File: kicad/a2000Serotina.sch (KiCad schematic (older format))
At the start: 23 parts

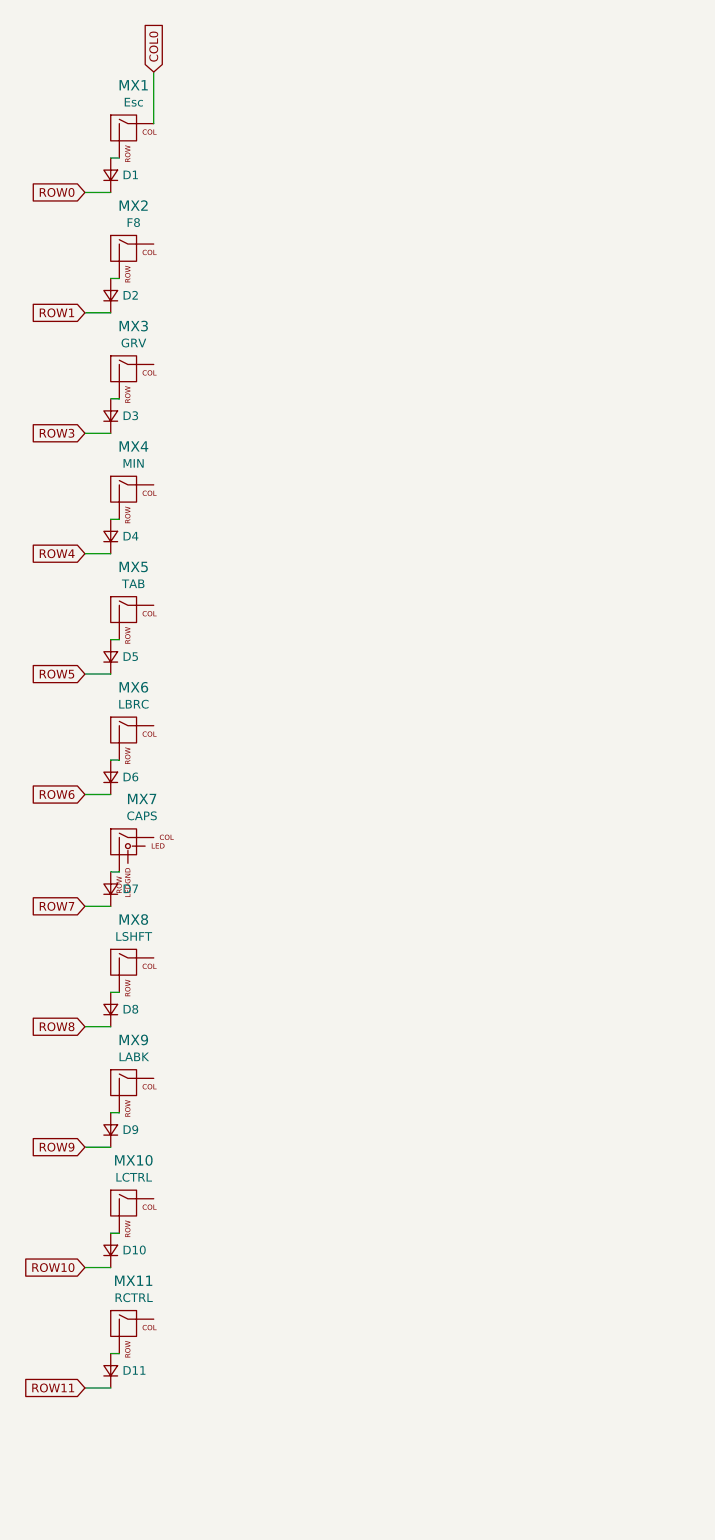
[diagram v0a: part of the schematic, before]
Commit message: Further work on Keyboard Matrix
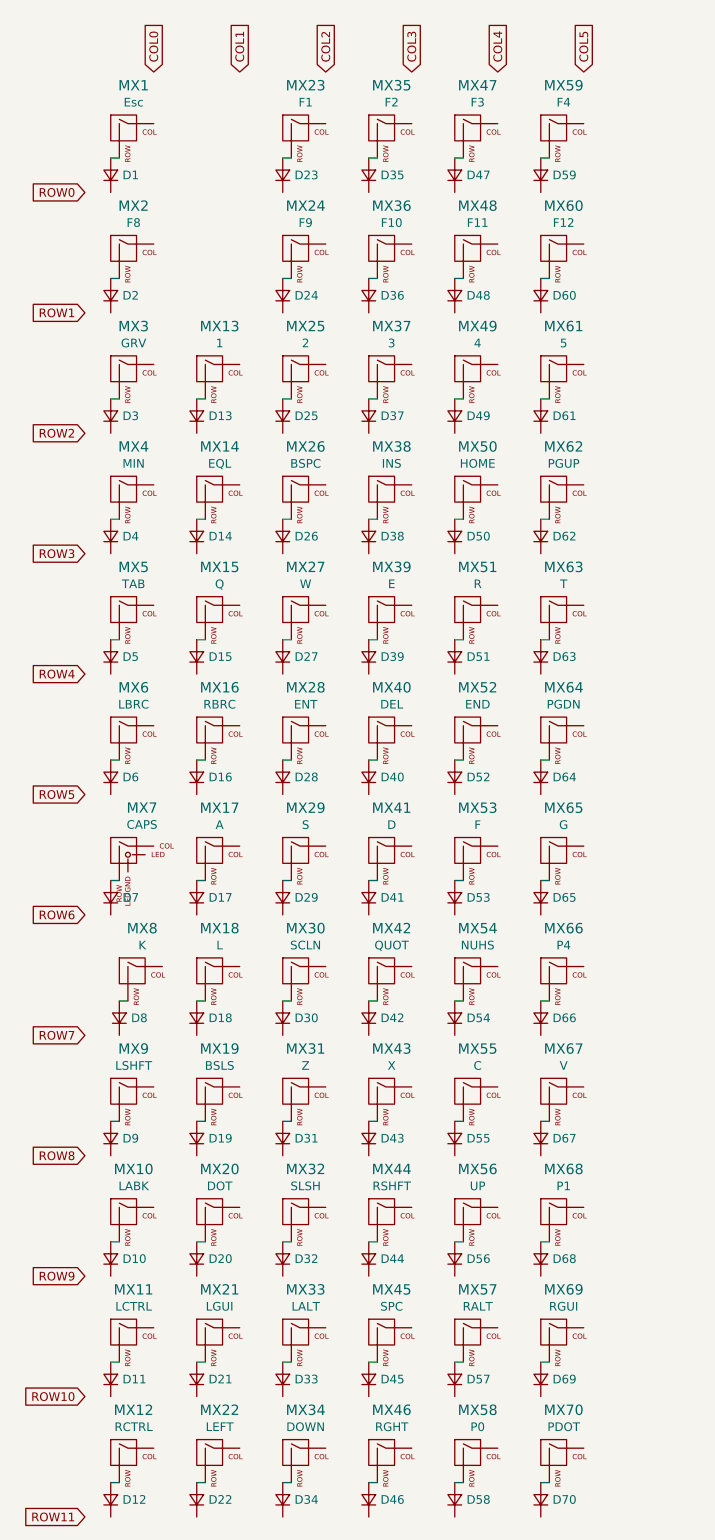
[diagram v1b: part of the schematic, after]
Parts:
- added D13, D14, D15, D16, D17, D18, D19, D20, D21, D22, D23, D24, D25, D26, D27, D28, D29, D30, D31, D32, D33, D34, D35, D36, D37, D38, D39, D40, D41, D42, D43, D44, D45, D46, D47, D48, D49, D50, D51, D52, D53, D54, D55, D56, D57, D58, D59, D60, D61, D62, D63, D64, D65, D66, D67, D68, D69, D70, D8: D_Small, symbol Device:D_Small
- added MX13, MX14, MX15, MX16, MX17, MX18, MX19, MX20, MX21, MX22, MX23, MX24, MX25, MX26, MX27, MX28, MX29, MX30, MX31, MX32, MX33, MX34, MX35, MX36, MX37, MX38, MX39, MX40, MX41, MX42, MX43, MX44, MX45, MX46, MX47, MX48, MX49, MX50, MX51, MX52, MX53, MX54, MX55, MX56, MX57, MX58, MX59, MX60, MX61, MX62, MX63, MX64, MX65, MX66, MX67, MX68, MX69, MX70, MX8: MX-NoLED, symbol MX_Alps_Hybrid:MX-NoLED
- renumbered D9 to D10, D10 to D11, D11 to D12, D8 to D9, MX9 to MX10, MX10 to MX11, MX11 to MX12, MX8 to MX9
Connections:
- net COL0: no longer MX1.1 (COL)
- net ROW0: no longer D1.1 (K)
- net ROW1: no longer D2.1 (K)
- net ROW10: no longer D11.1 (K)
- net ROW11: no longer D12.1 (K)
- net ROW3: no longer D3.1 (K)
- net ROW4: no longer D4.1 (K)
- net ROW5: no longer D5.1 (K)
- net ROW6: no longer D6.1 (K)
- net ROW7: no longer D7.1 (K)
- net ROW8: no longer D9.1 (K)
- net ROW9: no longer D10.1 (K)
- new net: D13.2 (A), MX13.2 (ROW)
- new net: D14.2 (A), MX14.2 (ROW)
- new net: D15.2 (A), MX15.2 (ROW)
- new net: D16.2 (A), MX16.2 (ROW)
- new net: D17.2 (A), MX17.2 (ROW)
- new net: D19.2 (A), MX19.2 (ROW)
- new net: D20.2 (A), MX20.2 (ROW)
- new net: D21.2 (A), MX21.2 (ROW)
- new net: D22.2 (A), MX22.2 (ROW)
- new net: D25.2 (A), MX25.2 (ROW)
- new net: D24.2 (A), MX24.2 (ROW)
- new net: D23.2 (A), MX23.2 (ROW)
- new net: D26.2 (A), MX26.2 (ROW)
- new net: D27.2 (A), MX27.2 (ROW)
- new net: D28.2 (A), MX28.2 (ROW)
- new net: D29.2 (A), MX29.2 (ROW)
- new net: D30.2 (A), MX30.2 (ROW)
- new net: D31.2 (A), MX31.2 (ROW)
- new net: D18.2 (A), MX18.2 (ROW)
- new net: D8.2 (A), MX8.2 (ROW)
- new net: D32.2 (A), MX32.2 (ROW)
- new net: D33.2 (A), MX33.2 (ROW)
- new net: D34.2 (A), MX34.2 (ROW)
- new net: D35.2 (A), MX35.2 (ROW)
- new net: D36.2 (A), MX36.2 (ROW)
- new net: D37.2 (A), MX37.2 (ROW)
- new net: D38.2 (A), MX38.2 (ROW)
- new net: D39.2 (A), MX39.2 (ROW)
- new net: D40.2 (A), MX40.2 (ROW)
- new net: D41.2 (A), MX41.2 (ROW)
- new net: D42.2 (A), MX42.2 (ROW)
- new net: D43.2 (A), MX43.2 (ROW)
- new net: D44.2 (A), MX44.2 (ROW)
- new net: D45.2 (A), MX45.2 (ROW)
- new net: D46.2 (A), MX46.2 (ROW)
- new net: D47.2 (A), MX47.2 (ROW)
- new net: D48.2 (A), MX48.2 (ROW)
- new net: D49.2 (A), MX49.2 (ROW)
- new net: D50.2 (A), MX50.2 (ROW)
- new net: D51.2 (A), MX51.2 (ROW)
- new net: D52.2 (A), MX52.2 (ROW)
- new net: D53.2 (A), MX53.2 (ROW)
- new net: D54.2 (A), MX54.2 (ROW)
- new net: D55.2 (A), MX55.2 (ROW)
- new net: D56.2 (A), MX56.2 (ROW)
- new net: D57.2 (A), MX57.2 (ROW)
- new net: D58.2 (A), MX58.2 (ROW)
- new net: D59.2 (A), MX59.2 (ROW)
- new net: D60.2 (A), MX60.2 (ROW)
- new net: D61.2 (A), MX61.2 (ROW)
- new net: D62.2 (A), MX62.2 (ROW)
- new net: D63.2 (A), MX63.2 (ROW)
- new net: D64.2 (A), MX64.2 (ROW)
- new net: D65.2 (A), MX65.2 (ROW)
- new net: D66.2 (A), MX66.2 (ROW)
- new net: D67.2 (A), MX67.2 (ROW)
- new net: D68.2 (A), MX68.2 (ROW)
- new net: D69.2 (A), MX69.2 (ROW)
- new net: D70.2 (A), MX70.2 (ROW)
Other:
- moved on the sheet: D10, D11, D12, D7, D9, MX10, MX11, MX12, MX7, MX9

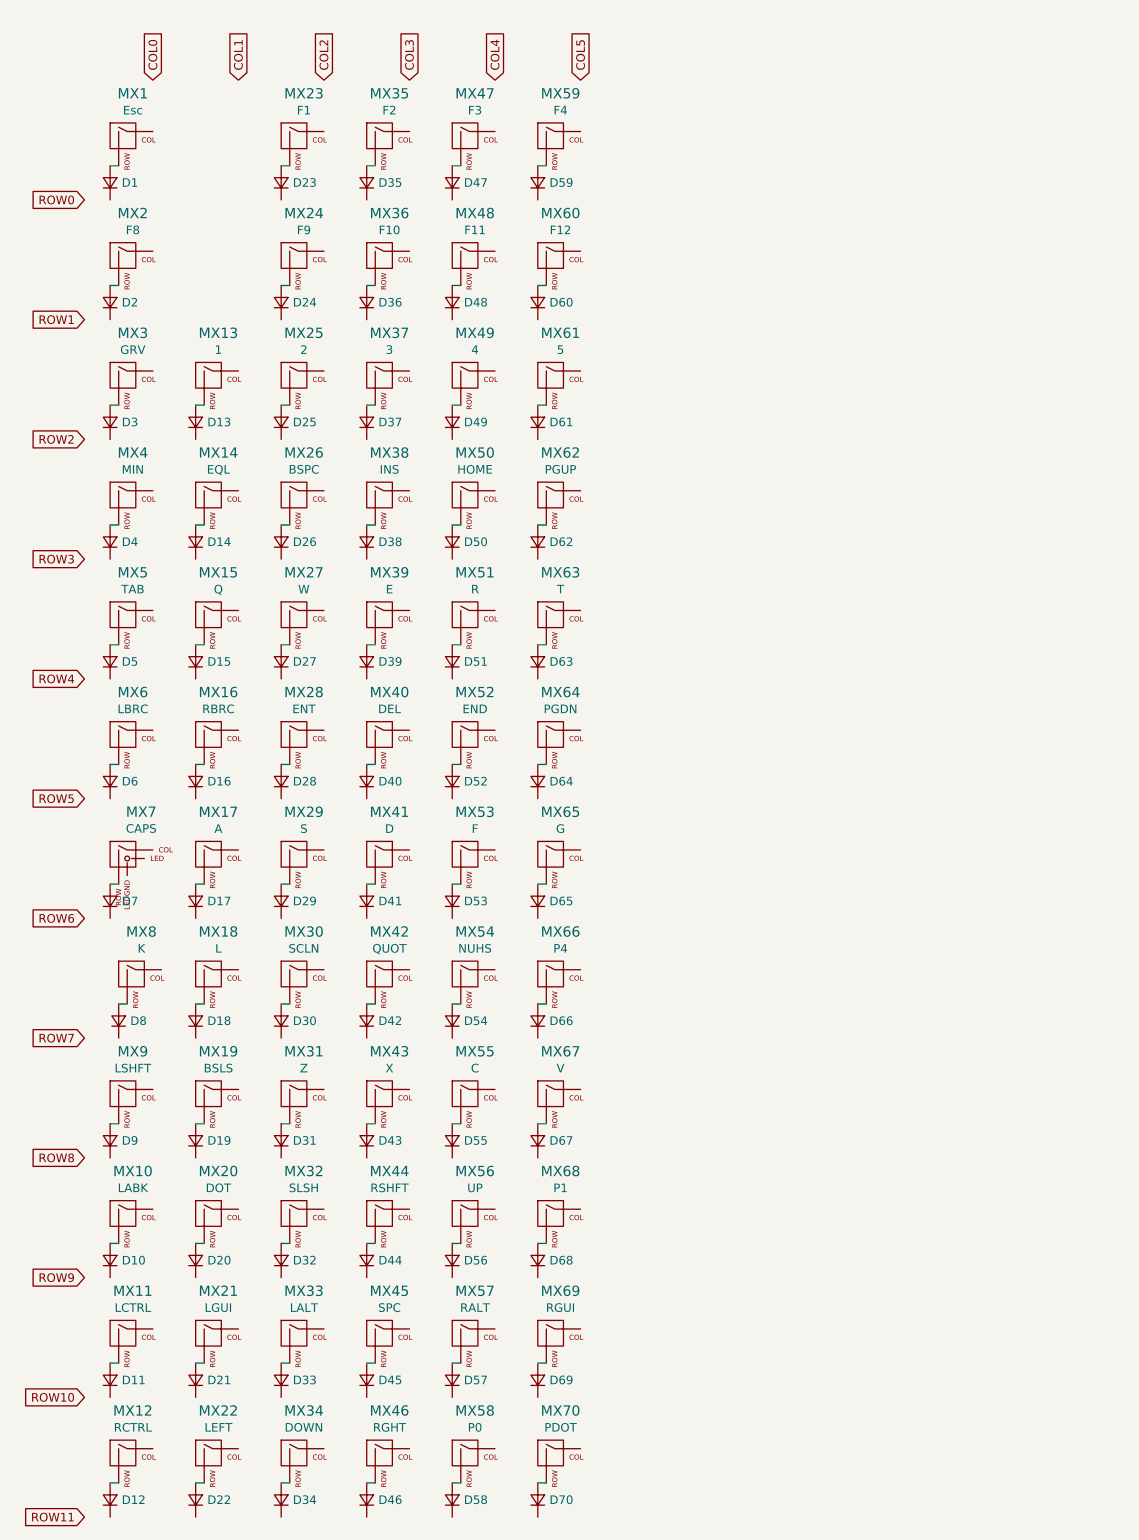
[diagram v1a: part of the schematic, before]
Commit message: Matrix now complete.
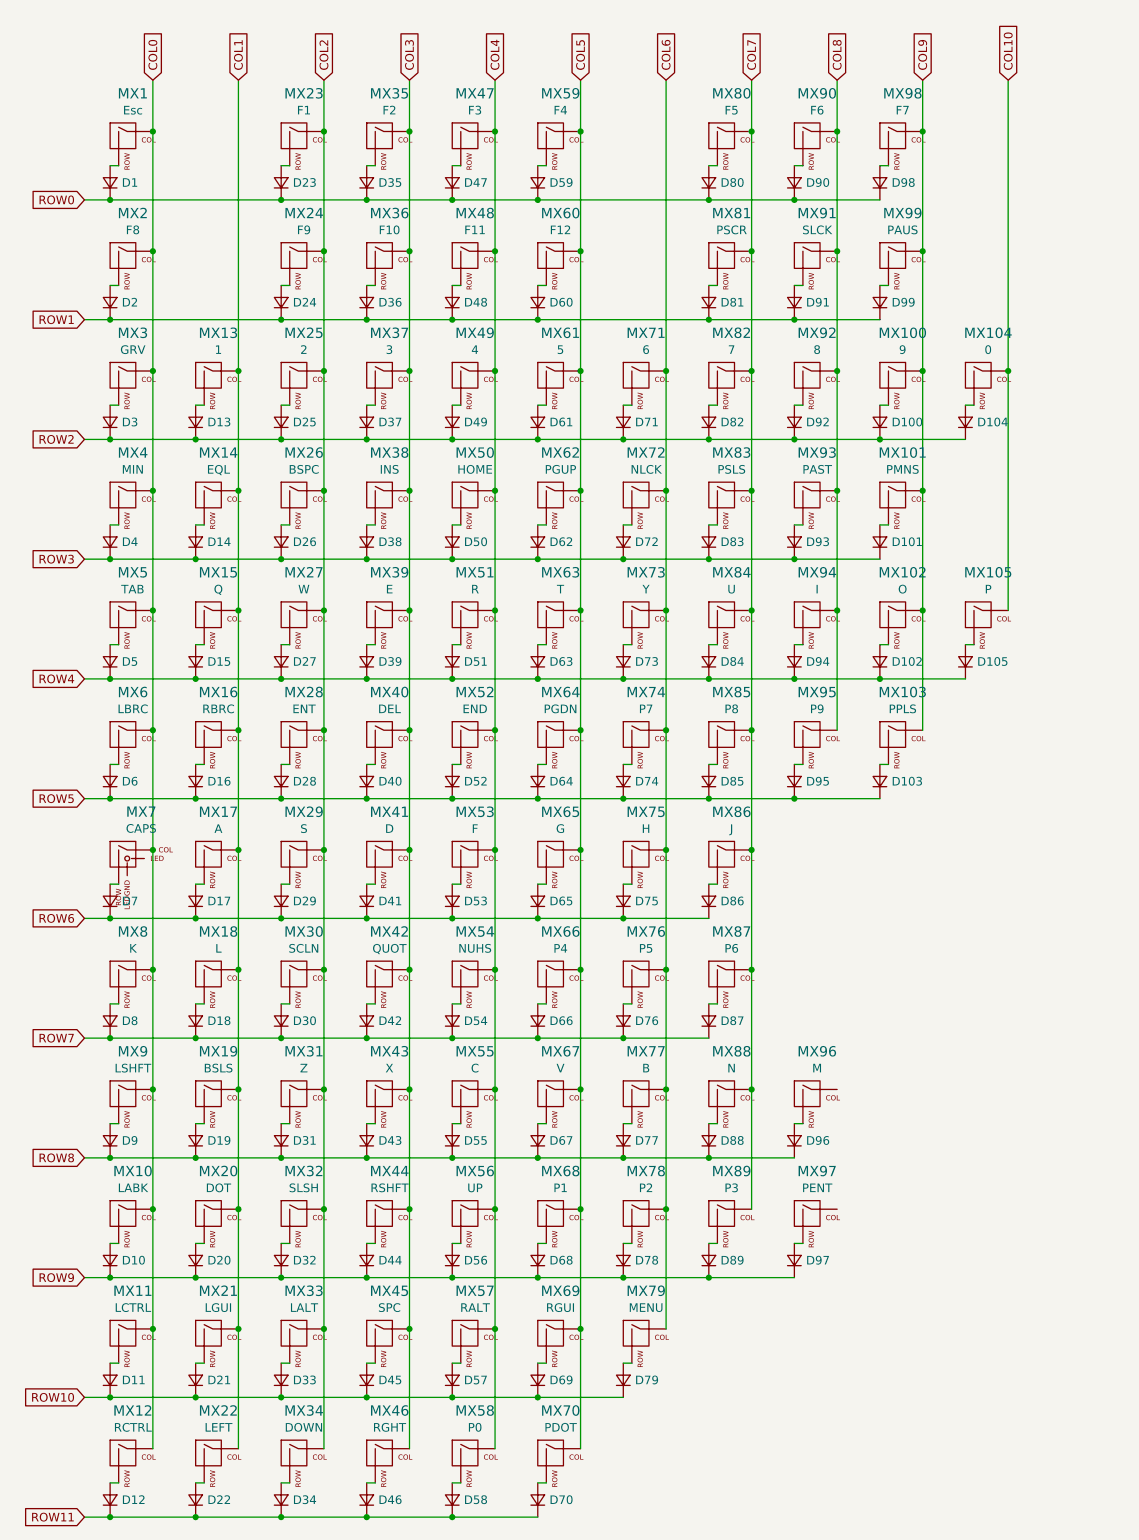
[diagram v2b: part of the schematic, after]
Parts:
- added D100, D101, D102, D103, D104, D105, D71, D72, D73, D74, D75, D76, D77, D78, D79, D80, D81, D82, D83, D84, D85, D86, D87, D88, D89, D90, D91, D92, D93, D94, D95, D96, D97, D98, D99: D_Small, symbol Device:D_Small
- added MX100, MX101, MX102, MX103, MX104, MX105, MX71, MX72, MX73, MX74, MX75, MX76, MX77, MX78, MX79, MX80, MX81, MX82, MX83, MX84, MX85, MX86, MX87, MX88, MX89, MX90, MX91, MX92, MX93, MX94, MX95, MX96, MX97, MX98, MX99: MX-NoLED, symbol MX_Alps_Hybrid:MX-NoLED
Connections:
- net COL0: now also MX1.1 (COL), MX10.1 (COL), MX11.1 (COL), MX12.1 (COL), MX2.1 (COL), MX3.1 (COL), MX4.1 (COL), MX5.1 (COL), MX6.1 (COL), MX7.1 (COL), MX8.1 (COL), MX9.1 (COL)
- net COL1: now also MX13.1 (COL), MX14.1 (COL), MX15.1 (COL), MX16.1 (COL), MX17.1 (COL), MX18.1 (COL), MX19.1 (COL), MX20.1 (COL), MX21.1 (COL), MX22.1 (COL)
- net COL10: now also MX104.1 (COL), MX105.1 (COL)
- net COL2: now also MX23.1 (COL), MX24.1 (COL), MX25.1 (COL), MX26.1 (COL), MX27.1 (COL), MX28.1 (COL), MX29.1 (COL), MX30.1 (COL), MX31.1 (COL), MX32.1 (COL), MX33.1 (COL), MX34.1 (COL)
- net COL3: now also MX35.1 (COL), MX36.1 (COL), MX37.1 (COL), MX38.1 (COL), MX39.1 (COL), MX40.1 (COL), MX41.1 (COL), MX42.1 (COL), MX43.1 (COL), MX44.1 (COL), MX45.1 (COL), MX46.1 (COL)
- net COL4: now also MX47.1 (COL), MX48.1 (COL), MX49.1 (COL), MX50.1 (COL), MX51.1 (COL), MX52.1 (COL), MX53.1 (COL), MX54.1 (COL), MX55.1 (COL), MX56.1 (COL), MX57.1 (COL), MX58.1 (COL)
- net COL5: now also MX59.1 (COL), MX60.1 (COL), MX61.1 (COL), MX62.1 (COL), MX63.1 (COL), MX64.1 (COL), MX65.1 (COL), MX66.1 (COL), MX67.1 (COL), MX68.1 (COL), MX69.1 (COL), MX70.1 (COL)
- net COL6: now also MX71.1 (COL), MX72.1 (COL), MX73.1 (COL), MX74.1 (COL), MX75.1 (COL), MX76.1 (COL), MX77.1 (COL), MX78.1 (COL), MX79.1 (COL)
- net COL7: now also MX80.1 (COL), MX81.1 (COL), MX82.1 (COL), MX83.1 (COL), MX84.1 (COL), MX85.1 (COL), MX86.1 (COL), MX87.1 (COL), MX88.1 (COL), MX89.1 (COL)
- net COL8: now also MX90.1 (COL), MX91.1 (COL), MX92.1 (COL), MX93.1 (COL), MX94.1 (COL), MX95.1 (COL)
- net COL9: now also MX100.1 (COL), MX101.1 (COL), MX102.1 (COL), MX103.1 (COL), MX98.1 (COL), MX99.1 (COL)
- net ROW0: now also D1.1 (K), D23.1 (K), D35.1 (K), D47.1 (K), D59.1 (K), D80.1 (K), D90.1 (K), D98.1 (K)
- net ROW1: now also D2.1 (K), D24.1 (K), D36.1 (K), D48.1 (K), D60.1 (K), D81.1 (K), D91.1 (K), D99.1 (K)
- net ROW10: now also D11.1 (K), D21.1 (K), D33.1 (K), D45.1 (K), D57.1 (K), D69.1 (K), D79.1 (K)
- net ROW11: now also D12.1 (K), D22.1 (K), D34.1 (K), D46.1 (K), D58.1 (K), D70.1 (K)
- net ROW2: now also D13.1 (K), D25.1 (K), D3.1 (K), D37.1 (K), D49.1 (K), D61.1 (K), D100.1 (K), D104.1 (K), D71.1 (K), D82.1 (K), D92.1 (K)
- net ROW3: now also D14.1 (K), D26.1 (K), D38.1 (K), D4.1 (K), D50.1 (K), D62.1 (K), D101.1 (K), D72.1 (K), D83.1 (K), D93.1 (K)
- net ROW4: now also D15.1 (K), D27.1 (K), D39.1 (K), D5.1 (K), D51.1 (K), D63.1 (K), D102.1 (K), D105.1 (K), D73.1 (K), D84.1 (K), D94.1 (K)
- net ROW5: now also D16.1 (K), D28.1 (K), D40.1 (K), D52.1 (K), D6.1 (K), D64.1 (K), D103.1 (K), D74.1 (K), D85.1 (K), D95.1 (K)
- net ROW6: now also D17.1 (K), D29.1 (K), D41.1 (K), D53.1 (K), D65.1 (K), D7.1 (K), D75.1 (K), D86.1 (K)
- net ROW7: now also D18.1 (K), D30.1 (K), D42.1 (K), D54.1 (K), D66.1 (K), D8.1 (K), D76.1 (K), D87.1 (K)
- net ROW8: now also D19.1 (K), D31.1 (K), D43.1 (K), D55.1 (K), D67.1 (K), D9.1 (K), D77.1 (K), D88.1 (K), D96.1 (K)
- net ROW9: now also D10.1 (K), D20.1 (K), D32.1 (K), D44.1 (K), D56.1 (K), D68.1 (K), D78.1 (K), D89.1 (K), D97.1 (K)
- new net: D71.2 (A), MX71.2 (ROW)
- new net: D72.2 (A), MX72.2 (ROW)
- new net: D73.2 (A), MX73.2 (ROW)
- new net: D74.2 (A), MX74.2 (ROW)
- new net: D75.2 (A), MX75.2 (ROW)
- new net: D76.2 (A), MX76.2 (ROW)
- new net: D77.2 (A), MX77.2 (ROW)
- new net: D78.2 (A), MX78.2 (ROW)
- new net: D79.2 (A), MX79.2 (ROW)
- new net: D80.2 (A), MX80.2 (ROW)
- new net: D81.2 (A), MX81.2 (ROW)
- new net: D82.2 (A), MX82.2 (ROW)
- new net: D83.2 (A), MX83.2 (ROW)
- new net: D84.2 (A), MX84.2 (ROW)
- new net: D85.2 (A), MX85.2 (ROW)
- new net: D86.2 (A), MX86.2 (ROW)
- new net: D87.2 (A), MX87.2 (ROW)
- new net: D88.2 (A), MX88.2 (ROW)
- new net: D89.2 (A), MX89.2 (ROW)
- new net: D90.2 (A), MX90.2 (ROW)
- new net: D91.2 (A), MX91.2 (ROW)
- new net: D92.2 (A), MX92.2 (ROW)
- new net: D93.2 (A), MX93.2 (ROW)
- new net: D94.2 (A), MX94.2 (ROW)
- new net: D95.2 (A), MX95.2 (ROW)
- new net: D96.2 (A), MX96.2 (ROW)
- new net: D97.2 (A), MX97.2 (ROW)
- new net: D98.2 (A), MX98.2 (ROW)
- new net: D99.2 (A), MX99.2 (ROW)
- new net: D100.2 (A), MX100.2 (ROW)
- new net: D101.2 (A), MX101.2 (ROW)
- new net: D102.2 (A), MX102.2 (ROW)
- new net: D103.2 (A), MX103.2 (ROW)
- new net: D104.2 (A), MX104.2 (ROW)
- new net: D105.2 (A), MX105.2 (ROW)
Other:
- moved on the sheet: D8, MX8
